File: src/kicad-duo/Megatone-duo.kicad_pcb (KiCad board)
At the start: 2 copper layers, 28.4 x 27.4 mm, 22 parts, among them P1 Classic, P2 Boost, P3 Gnd, SW1 LORLIN_2X6

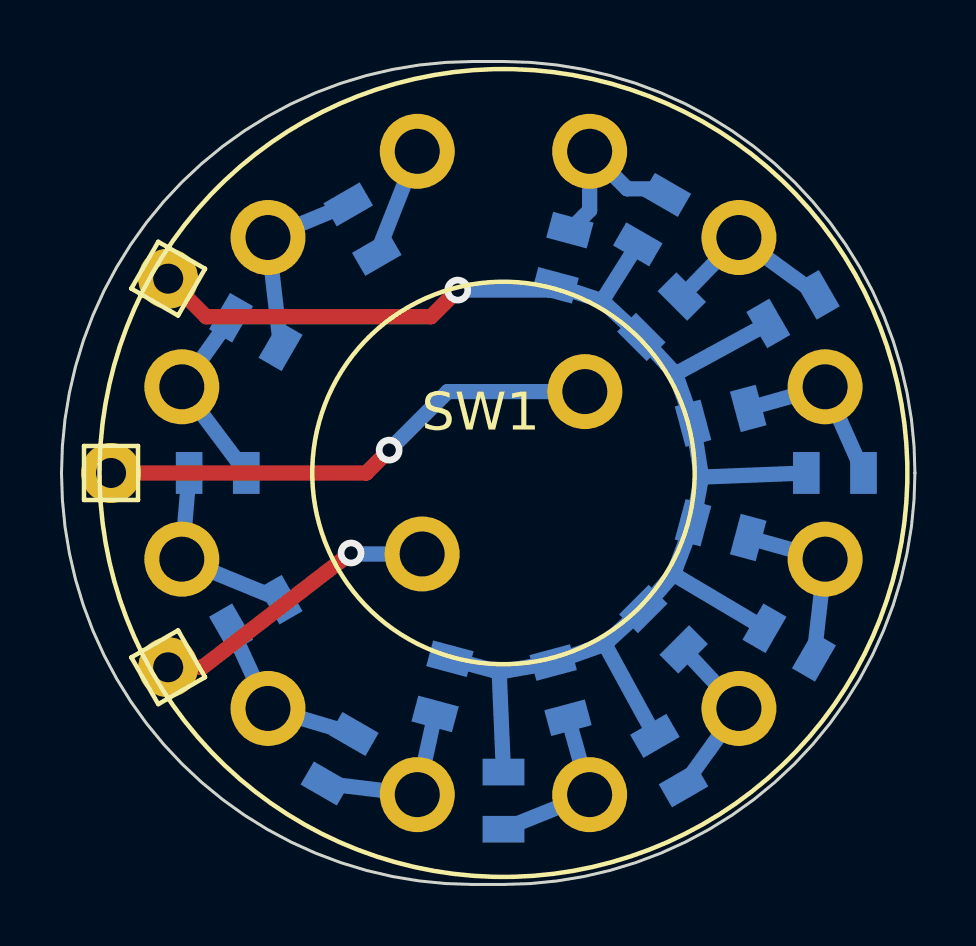
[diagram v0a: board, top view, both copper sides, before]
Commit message: plots for v6.2
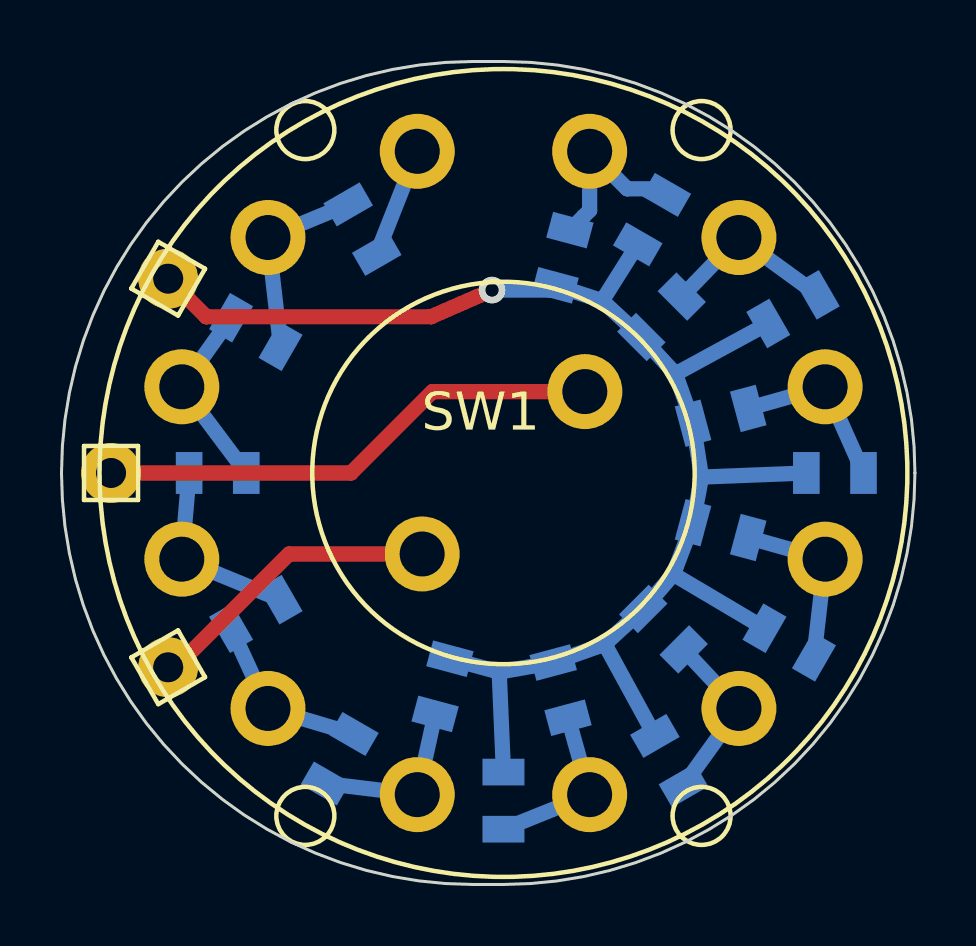
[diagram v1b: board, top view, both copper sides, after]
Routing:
- net Net-(P2-Pad1): track 17.2 -> 16.9 mm, vias 1 -> 0
- net Net-(P1-Pad1): track 9.78 -> 10.0 mm, vias 1 -> 0
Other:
- board text added: "Megatone DUO 6.2"
- board text removed: "megatone DUO 6.2"
- board text removed: "v 6.1"
